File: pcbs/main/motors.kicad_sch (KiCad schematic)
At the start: 80 parts, among them J4 Jumpers, M1 FRONT_LEFT_MOTOR, M2 BACK_LEFT_MOTOR, M3 BACK_RIGHT_MOTOR, M4 FRONT_RIGHT_MOTOR, Q1 2SC945, Q2 2SC945, Q3 2SC945, Q4 2SC945, Q5 2SC945, Q6 2SC945, Q7 2SC945, Q8 2SC945

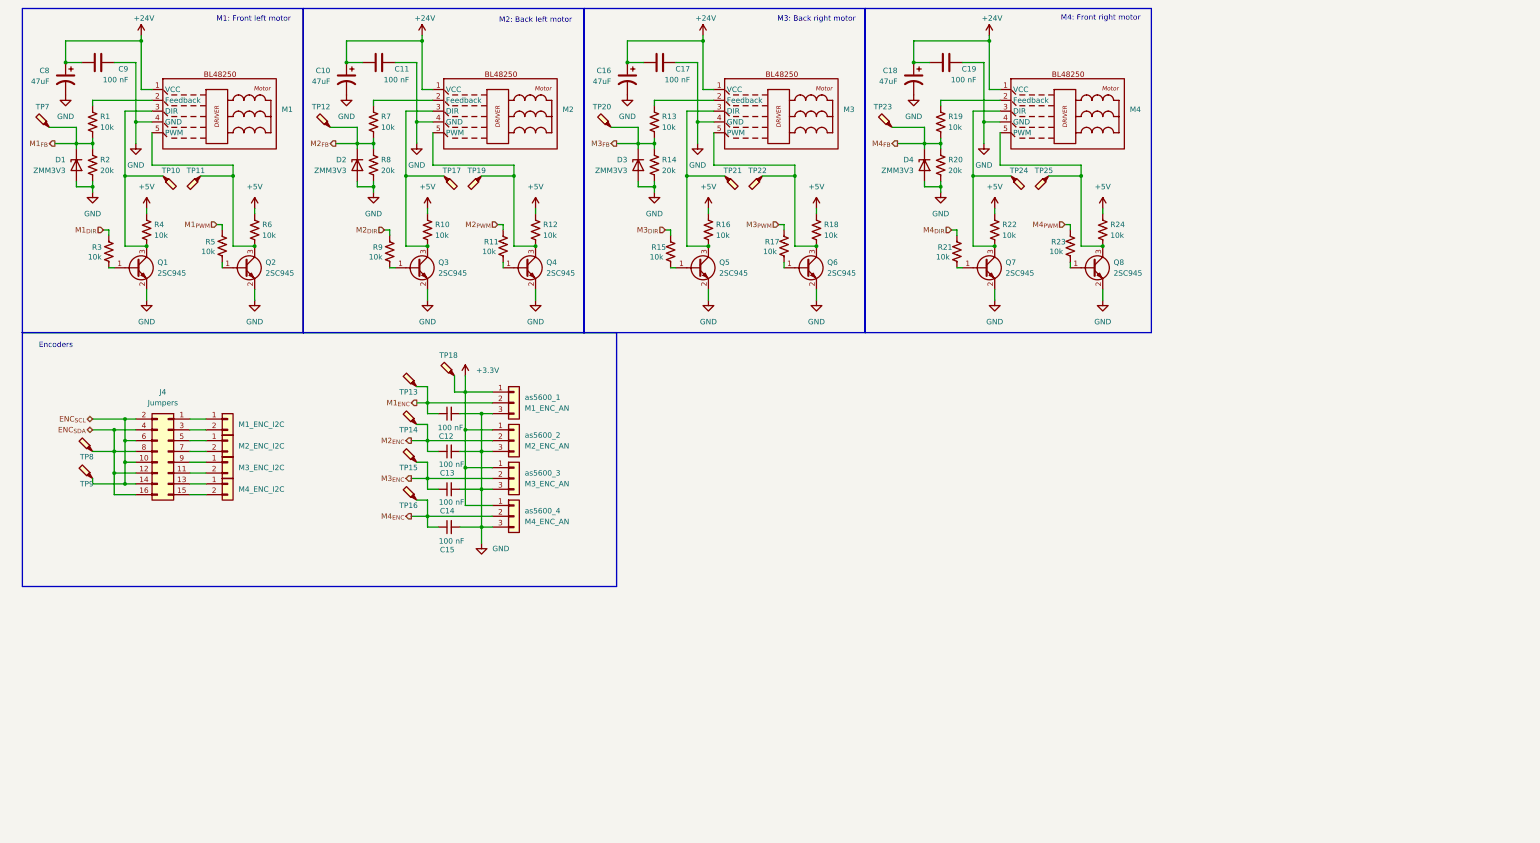
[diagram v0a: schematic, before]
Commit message: Final rev. V02 main board
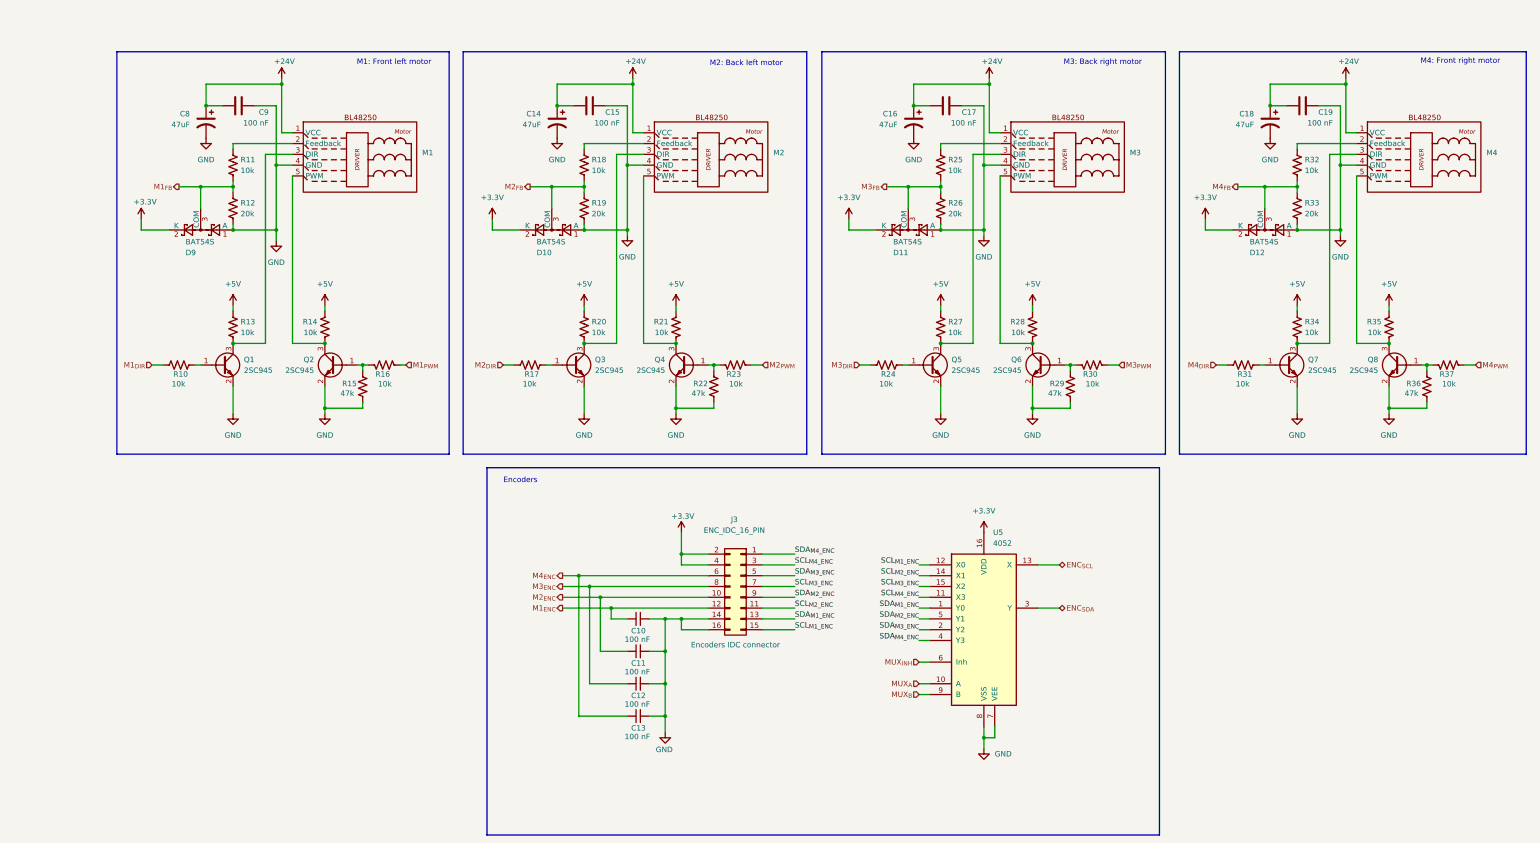
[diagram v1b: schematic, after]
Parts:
- removed C14, C15: 100 nF, Capacitor_SMD:C_0603_1608Metric, symbol Device:C_Small
- removed D1, D2, D3, D4: ZMM3V3, Diode_SMD:D_MiniMELF, symbol Diode:ZMMxx
- removed J4: Jumpers, Connector_PinHeader_2.54mm:PinHeader_2x08_P2.54mm_Vertical, symbol Connector_Generic:Conn_02x08_Odd_Even
- removed R10, R11, R12, R16, R18, R9: 10k, Resistor_SMD:R_0603_1608Metric, symbol Device:R_US
- removed TP10: M1_DIR_Probe, TestPoint:TestPoint_Pad_D1.0mm, symbol Connector:TestPoint_Probe
- removed TP11: M1_PWM_Probe, TestPoint:TestPoint_Loop_D2.50mm_Drill1.0mm_LowProfile, symbol Connector:TestPoint_Probe
- removed TP12: M2_FB_Probe, TestPoint:TestPoint_Loop_D2.50mm_Drill1.0mm_LowProfile, symbol Connector:TestPoint_Probe
- removed TP13: M1_ENC_Probe, TestPoint:TestPoint_Loop_D2.50mm_Drill1.0mm_LowProfile, symbol Connector:TestPoint_Probe
- removed TP14: M2_ENC_Probe, TestPoint:TestPoint_Loop_D2.50mm_Drill1.0mm_LowProfile, symbol Connector:TestPoint_Probe
- removed TP15: M3_ENC_Probe, TestPoint:TestPoint_Loop_D2.50mm_Drill1.0mm_LowProfile, symbol Connector:TestPoint_Probe
- removed TP16: M4_ENC_Probe, TestPoint:TestPoint_Loop_D2.50mm_Drill1.0mm_LowProfile, symbol Connector:TestPoint_Probe
- removed TP17: M2_DIR_Probe, TestPoint:TestPoint_Pad_D1.0mm, symbol Connector:TestPoint_Probe
- removed TP18: ENC_VCC_Probe, TestPoint:TestPoint_Pad_D1.0mm, symbol Connector:TestPoint_Probe
- removed TP19: M2_PWM_Probe, TestPoint:TestPoint_Loop_D2.50mm_Drill1.0mm_LowProfile, symbol Connector:TestPoint_Probe
- removed TP20: M3_FB_Probe, TestPoint:TestPoint_Loop_D2.50mm_Drill1.0mm_LowProfile, symbol Connector:TestPoint_Probe
- removed TP21: M3_DIR_Probe, TestPoint:TestPoint_Pad_D1.0mm, symbol Connector:TestPoint_Probe
- removed TP22: M3_PWM_Probe, TestPoint:TestPoint_Loop_D2.50mm_Drill1.0mm_LowProfile, symbol Connector:TestPoint_Probe
- removed TP23: M4_FB_Probe, TestPoint:TestPoint_Loop_D2.50mm_Drill1.0mm_LowProfile, symbol Connector:TestPoint_Probe
- removed TP24: M4_DIR_Probe, TestPoint:TestPoint_Pad_D1.0mm, symbol Connector:TestPoint_Probe
- removed TP25: M4_PWM_Probe, TestPoint:TestPoint_Loop_D2.50mm_Drill1.0mm_LowProfile, symbol Connector:TestPoint_Probe
- removed TP7: M1_FB_Probe, TestPoint:TestPoint_Loop_D2.50mm_Drill1.0mm_LowProfile, symbol Connector:TestPoint_Probe
- removed TP8: ENC_SDA_Probe, TestPoint:TestPoint_Loop_D2.50mm_Drill1.0mm_LowProfile, symbol Connector:TestPoint_Probe
- removed TP9: ENC_SCL_Probe, TestPoint:TestPoint_Loop_D2.50mm_Drill1.0mm_LowProfile, symbol Connector:TestPoint_Probe
- removed as1: M1_ENC_I2C, Connector_JST:JST_XH_B2B-XH-A_1x02_P2.50mm_Vertical, symbol Connector_Generic:Conn_01x02
- removed as2: M2_ENC_I2C, Connector_JST:JST_XH_B2B-XH-A_1x02_P2.50mm_Vertical, symbol Connector_Generic:Conn_01x02
- removed as3: M3_ENC_I2C, Connector_JST:JST_XH_B2B-XH-A_1x02_P2.50mm_Vertical, symbol Connector_Generic:Conn_01x02
- removed as4: M4_ENC_I2C, Connector_JST:JST_XH_B2B-XH-A_1x02_P2.50mm_Vertical, symbol Connector_Generic:Conn_01x02
- removed as5600_1: M1_ENC_AN, Connector_JST:JST_XH_B3B-XH-A_1x03_P2.50mm_Vertical, symbol Connector_Generic:Conn_01x03
- removed as5600_2: M2_ENC_AN, Connector_JST:JST_XH_B3B-XH-A_1x03_P2.50mm_Vertical, symbol Connector_Generic:Conn_01x03
- removed as5600_3: M3_ENC_AN, Connector_JST:JST_XH_B3B-XH-A_1x03_P2.50mm_Vertical, symbol Connector_Generic:Conn_01x03
- removed as5600_4: M4_ENC_AN, Connector_JST:JST_XH_B3B-XH-A_1x03_P2.50mm_Vertical, symbol Connector_Generic:Conn_01x03
- added C10, C11: 100 nF, Capacitor_SMD:C_0603_1608Metric, symbol Device:C_Small
- added D10, D11, D12, D9: BAT54S, Package_TO_SOT_SMD:SOT-23, symbol Diode:BAT54S
- added J3: ENC_IDC_16_PIN, Connector_IDC:IDC-Header_2x08_P2.54mm_Vertical, symbol Connector_Generic:Conn_02x08_Odd_Even
- added R20, R27, R28, R30, R31, R34, R35, R37: 10k, Resistor_SMD:R_0603_1608Metric, symbol Device:R_US
- added R29, R36: 47k, Resistor_SMD:R_0603_1608Metric, symbol Device:R_US
- added U5: 4052, Package_DIP:DIP-16_W7.62mm, symbol 4xxx:4052
- R15, R22: value 10k -> 47k
- renumbered C10 to C14, C11 to C15, R3 to R10, R1 to R11, R2 to R12, R4 to R13, R6 to R14, R5 to R16, R7 to R18, R8 to R19, R13 to R25, R14 to R26, R19 to R32, R20 to R33
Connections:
- net +3.3V: now also D10.2 (K), D11.2 (K), D12.2 (K), D9.2 (K), J3.2 (Pin_2), J3.4 (Pin_4), U5.16 (VDD)
- net +5V: now also R21.2, R20.2, R27.2, R28.2, R34.2, R35.2; no longer R22.2, R24.2
- net ENC_{SCL}: now also U5.13 (X)
- net ENC_{SDA}: now also U5.3 (Y)
- net GND: now also R15.2, R22.2, C10.2, C11.2, D10.1 (A), D11.1 (A), D12.1 (A), D9.1 (A), J3.14 (Pin_14), J3.16 (Pin_16), R29.2, R36.2, U5.7 (VEE), U5.8 (VSS)
- net M1_{ENC}: now also C10.1, J3.12 (Pin_12); no longer C12.1
- net M1_{FB}: now also D9.3 (COM)
- net M2_{DIR}: now also R17.1
- net M2_{ENC}: now also C11.1, J3.10 (Pin_10); no longer C13.1
- net M2_{FB}: now also D10.3 (COM)
- net M2_{PWM}: now also R23.1
- net M3_{DIR}: now also R24.1; no longer R15.1
- net M3_{ENC}: now also C12.1, J3.8 (Pin_8)
- net M3_{FB}: now also D11.3 (COM)
- net M3_{PWM}: now also R30.1; no longer R17.1
- net M4_{DIR}: now also R31.1; no longer R21.1
- net M4_{ENC}: now also C13.1, J3.6 (Pin_6)
- net M4_{FB}: now also D12.3 (COM)
- net M4_{PWM}: now also R37.1; no longer R23.1
- net at M3.3 (DIR), Q5.3 (C): now also R27.1
- net at Q2.1 (B), R16.2: now also R15.1
- net at M3.5 (PWM), Q6.3 (C): now also R28.1
- net at R23.2: now also Q4.1 (B), R22.1; no longer Q8.1 (B)
- net at M2.3 (DIR), Q3.3 (C): now also R20.1
- net at M2.5 (PWM), Q4.3 (C): now also R21.1
- net at Q7.1 (B): now also R31.2; no longer R21.2
- net at Q3.1 (B): now also R17.2
- net at Q5.1 (B): now also R24.2; no longer R15.2
- net at Q6.1 (B): now also R29.1, R30.2; no longer R17.2
- net at M4.5 (PWM), Q8.3 (C): now also R35.1; no longer R24.1
- net at M4.3 (DIR), Q7.3 (C): now also R34.1; no longer R22.1
- new net: Q8.1 (B), R36.1, R37.2
- new net MUX_{A}: U5.10 (A)
- new net MUX_{B}: U5.9 (B)
- new net MUX_{INH}: U5.6 (Inh)
- new net SCL_{M1_ENC}: J3.15 (Pin_15), U5.12 (X0)
- new net SCL_{M2_ENC}: J3.11 (Pin_11), U5.14 (X1)
- new net SCL_{M3_ENC}: J3.7 (Pin_7), U5.15 (X2)
- new net SCL_{M4_ENC}: J3.3 (Pin_3), U5.11 (X3)
- new net SDA_{M1_ENC}: J3.13 (Pin_13), U5.1 (Y0)
- new net SDA_{M2_ENC}: J3.9 (Pin_9), U5.5 (Y1)
- new net SDA_{M3_ENC}: J3.5 (Pin_5), U5.2 (Y2)
- new net SDA_{M4_ENC}: J3.1 (Pin_1), U5.4 (Y3)
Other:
- moved on the sheet: C14, C15, C16, C17, C18, C19, C8, C9, M1, M2, M3, M4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
